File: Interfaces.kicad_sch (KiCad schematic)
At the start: 10 parts, among them J5 I2C1_Headers, J6 I/O_Headers_1

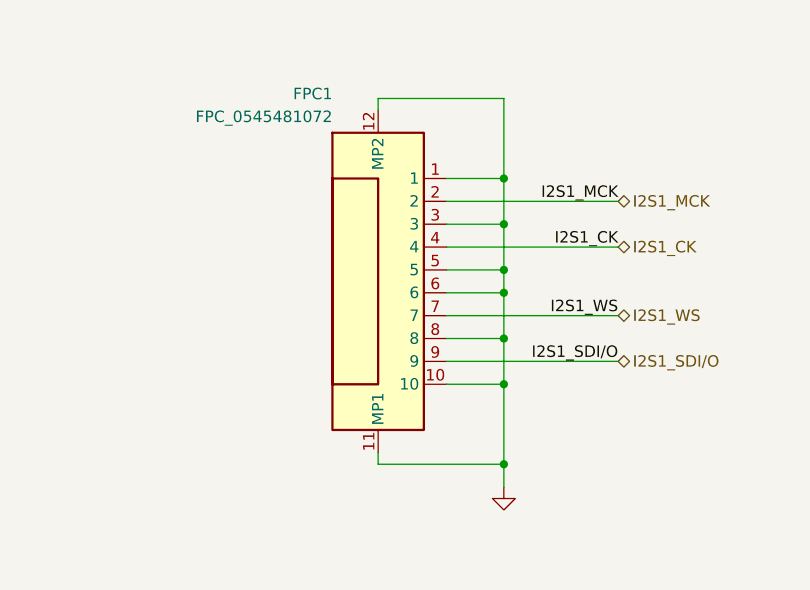
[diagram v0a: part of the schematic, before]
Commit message: Update
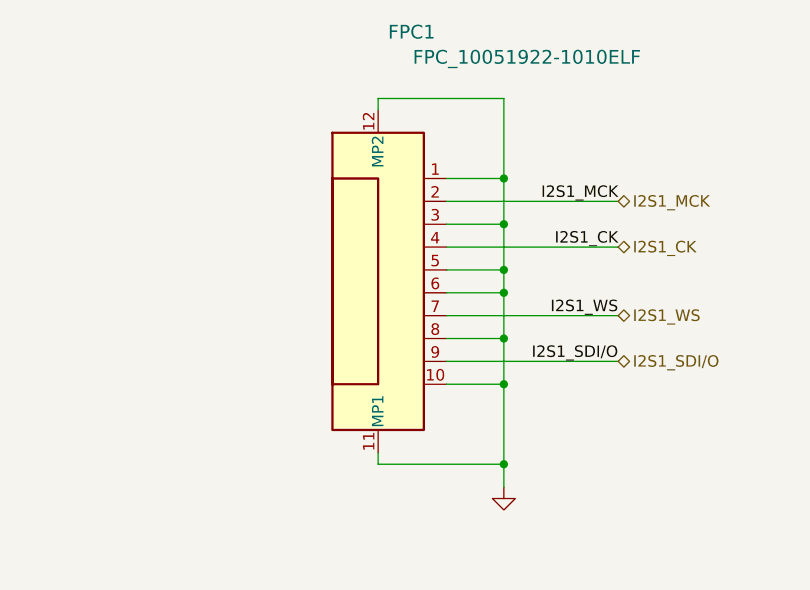
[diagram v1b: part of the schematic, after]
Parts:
- removed FPC1: FPC_0545481072, Personal_Project:FPC_0545481072, symbol Personal_Projects:FPC_0545481072
- added FPC1: FPC_10051922-1010ELF, Personal_Project:FPC_10051922_1010, symbol Personal_Projects:FPC_10051922-1010ELF
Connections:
- net GND: now also FPC1.1, FPC1.10, FPC1.11 (MP1), FPC1.12 (MP2), FPC1.3, FPC1.5, FPC1.6, FPC1.8
- net I2S1_CK: now also FPC1.4
- net I2S1_MCK: now also FPC1.2
- net I2S1_SDI/O: now also FPC1.9
- net I2S1_WS: now also FPC1.7
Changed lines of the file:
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@@
 	)
 	(symbol
-		(lib_id "Personal_Projects:FPC_0545481072")
+		(lib_id "Personal_Projects:FPC_10051922-1010ELF")
 		(at 172.72 52.07 0)
 		(unit 1)
@@
 		(dnp no)
 		(property "Reference" "FPC1"
-			(at 172.72 42.672 0)
+			(at 184.15 35.814 0)
 			(effects
 				(font
-					(size 1.27 1.27)
+					(size 1.524 1.524)
 				)
 				(justify right)
 			)
 		)
-		(property "Value" "FPC_0545481072"
-			(at 172.72 45.212 0)
+		(property "Value" "FPC_10051922-1010ELF"
+			(at 207.01 38.608 0)
 			(effects
 				(font
-					(size 1.27 1.27)
+					(size 1.524 1.524)
 				)
 				(justify right)
 			)
 		)
-		(property "Footprint" "Personal_Project:FPC_0545481072"
-			(at 194.31 146.99 0)
+		(property "Footprint" "Personal_Project:FPC_10051922_1010"
+			(at 172.72 99.06 0)
 			(effects
 				(font
 					(size 1.27 1.27)
+					(italic yes)
 				)
-				(justify left top)
 				(hide yes)
 			)
 		)
-		(property "Datasheet" "https://www.molex.com/en-us/products/part-detail-pdf/545481072?display=pdf"
-			(at 194.31 246.99 0)
+		(property "Datasheet" "10051922-1010ELF"
+			(at 172.72 95.25 0)
 			(effects
 				(font
 					(size 1.27 1.27)
+					(italic yes)
 				)
-				(justify left top)
 				(hide yes)
 			)
 		)
-		(property "Description" "0.50mm Pitch Easy-On FFC/FPC Connector, 1.20mm Height, Right-Angle, Surface Mount, ZIF, Bottom Contact Style, 10 Circuits, Gold (Au) Plating"
-			(at 172.72 82.55 0)
+		(property "Description" ""
+			(at 185.42 52.07 0)
 			(effects
 				(font
@@
 			)
 		)
-		(property "Height" "1.3"
-			(at 194.31 446.99 0)
-			(effects
-				(font
-					(size 1.27 1.27)
-				)
-				(justify left top)
-				(hide yes)
-			)
+		(pin "6"
 		)
-		(property "Arrow Part Number" "0545481072"
-			(at 194.31 546.99 0)
-			(effects
-				(font
-					(size 1.27 1.27)
-				)
-				(justify left top)
-				(hide yes)
-			)
-		)
-		(property "Arrow Price/Stock" ""
-			(at 194.31 646.99 0)
-			(effects
-				(font
-					(size 1.27 1.27)
-				)
-				(justify left top)
-				(hide yes)
-			)
-		)
-		(property "Manufacturer_Name" "Molex"
-			(at 194.31 746.99 0)
-			(effects
-				(font
-					(size 1.27 1.27)
-				)
-				(justify left top)
-				(hide yes)
-			)
-		)
-		(property "Manufacturer_Part_Number" "0545481072"
-			(at 194.31 846.99 0)
-			(effects
-				(font
-					(size 1.27 1.27)
-				)
-				(justify left top)
-				(hide yes)
-			)
+		(pin "9"
 		)
 		(pin "4"
@@
 		(pin "7"
 		)
-		(pin "6"
+		(pin "2"
 		)
 		(pin "5"
 		)
-		(pin "2"
+		(pin "3"
 		)
 		(pin "8"
 		)
-		(pin "3"
+		(pin "12"
 		)
 		(pin "10"
 		)
-		(pin "12"
+		(pin "1"
 		)
 		(pin "11"
 		)
-		(pin "9"
-		)
-		(pin "1"
-		)
 		(instances
